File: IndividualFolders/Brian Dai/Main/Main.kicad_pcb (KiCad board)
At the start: 4 copper layers, 76.2 x 67.6 mm, 77 parts, among them J1 USB_B_Micro, J3 Conn_01x03, J4 Conn_01x03, J5 Conn_01x03, J6 Conn_01x03, SW1 SW_Push, SW2 SW_Push, U1 RP2350A-QFN60, U10 LM75B, U11 MCS1802GS-50-Z, U12 MCS1802GS-50-Z, U13 MCS1802GS-50-Z, U14 LM2575-3.3BT, U2 W25Q128JVS, U3 AMS1117-3.3, U4 MMC5983MA, U5 ICM-42688-P, U6 INA226, U7 KX134-1211, U8 MS5611-01BA, U9 MCS1802GS-50-Z, Y1 ABM8-272-T3

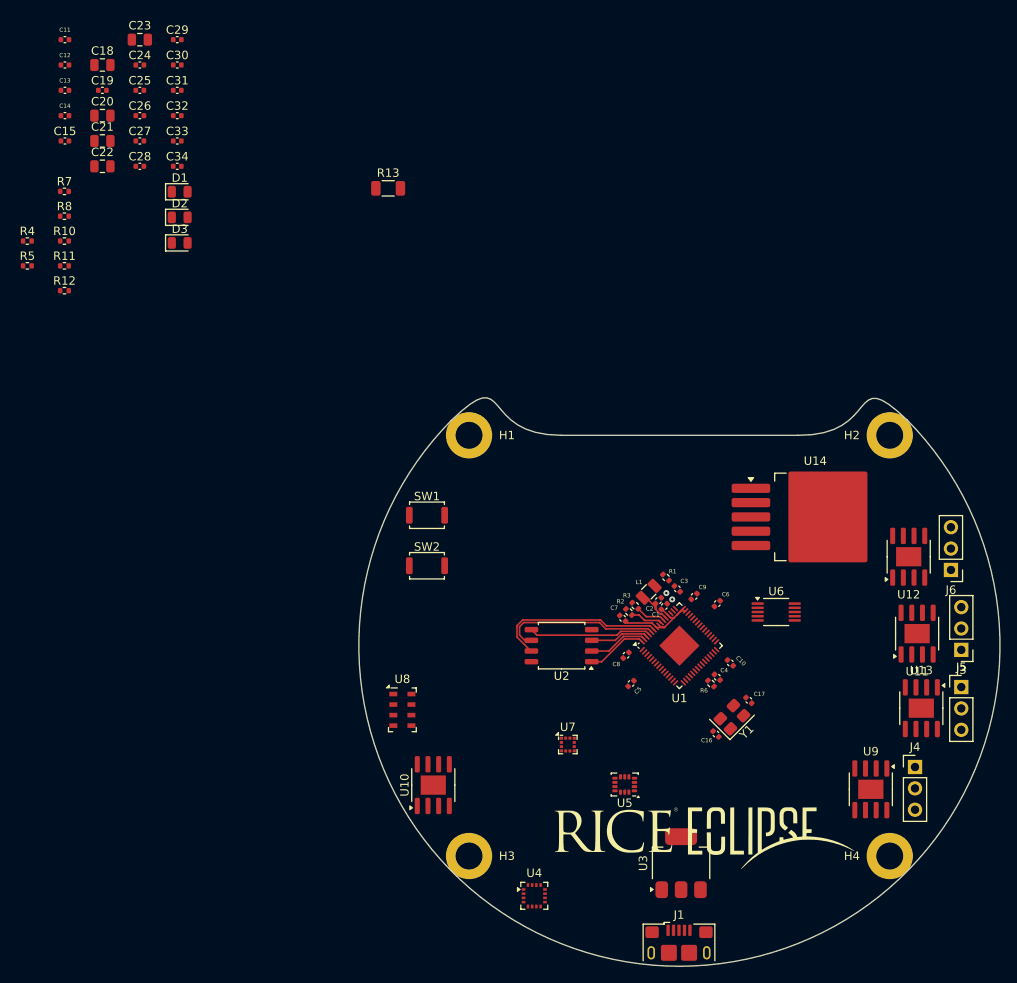
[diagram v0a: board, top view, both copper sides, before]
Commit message: Meeting 2/28/26
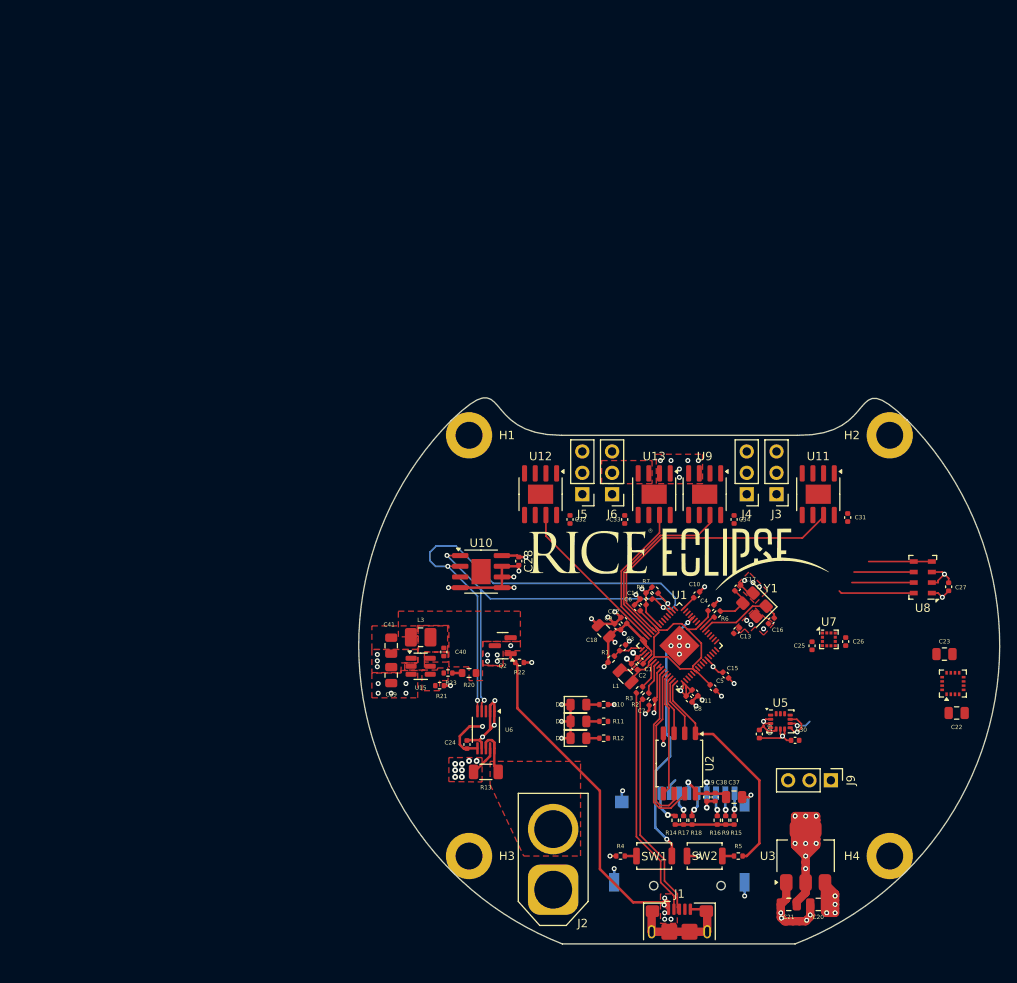
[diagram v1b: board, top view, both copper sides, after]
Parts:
- removed U14: LM2575-3.3BT, Package_TO_SOT_SMD:TO-263-5_TabPin3
- added C37: 10u, Capacitor_SMD:C_0805_2012Metric, F.Cu at (106.5, 118.0)
- added C38: 100n, Capacitor_SMD:C_0402_1005Metric, F.Cu at (104.2, 118.0)
- added C39: 10u, Capacitor_SMD:C_0805_2012Metric, F.Cu at (65.8, 103.5)
- added C40: 100n, Capacitor_SMD:C_0402_1005Metric, F.Cu at (72.0, 100.8)
- added C41: 22u, Capacitor_SMD:C_0805_2012Metric, F.Cu at (65.8, 100.0)
- added J2: XT60, Connector_AMASS:AMASS_XT60-M_1x02_P7.20mm_Vertical, F.Cu at (85.0, 129.0)
- added J7: MSD-4-A, otherComponents:CUI_MSD-4-A, B.Cu at (100.0, 125.3)
- added J9: Conn_01x03, Connector_PinHeader_2.54mm:PinHeader_1x03_P2.54mm_Vertical, F.Cu at (118.0, 116.0)
- added L3: 3.3u, Inductor_SMD:L_1008_2520Metric_Pad1.43x2.20mm_HandSolder, F.Cu at (69.2, 99.0)
- added Q2: Si2301CDS, Package_TO_SOT_SMD:SOT-23, F.Cu at (79.0, 100.0)
- added R14: 10k, Resistor_SMD:R_0402_1005Metric, F.Cu at (99.5, 120.8)
- added R15: 10k, Resistor_SMD:R_0402_1005Metric, F.Cu at (106.5, 120.8)
- added R16: 10k, Resistor_SMD:R_0402_1005Metric, F.Cu at (104.5, 120.8)
- added R17: 10k, Resistor_SMD:R_0402_1005Metric, F.Cu at (100.5, 120.8)
- added R18: 10k, Resistor_SMD:R_0402_1005Metric, F.Cu at (101.5, 120.8)
- added R20: 30k, Resistor_SMD:R_0603_1608Metric, F.Cu at (75.0, 103.2)
- added R21: 10k, Resistor_SMD:R_0402_1005Metric, F.Cu at (71.5, 104.8)
- added R22: 100k, Resistor_SMD:R_0402_1005Metric, F.Cu at (81.0, 102.0)
- added R23: 1k, Resistor_SMD:R_0402_1005Metric, F.Cu at (72.5, 103.2)
- added R9: 10k, Resistor_SMD:R_0402_1005Metric, F.Cu at (105.5, 120.8)
- added U15: AP62150WU, Package_TO_SOT_SMD:TSOT-23-6, F.Cu at (69.2, 102.5)
- D1: value LED -> RED_LED
- D2: value LED -> BLUE_LED
- D3: value LED -> GREEN_LED
- moved C20 126.6 mm to (116.5, 130.8), turned to 180 degrees
- moved C21 122.0 mm to (113.0, 130.8), turned to 180 degrees
- moved C22 120.5 mm to (132.9, 108.0), turned to 180 degrees
- moved C23 120.3 mm to (131.5, 101.0)
- moved C19 110.5 mm to (103.2, 118.0), turned to -90 degrees
- moved R5 109.8 mm to (107.0, 125.0)
- moved C27 109.8 mm to (132.0, 93.0), turned to 90 degrees
- moved C30 108.8 mm to (113.8, 111.2), turned to 180 degrees
- moved C11 107.8 mm to (101.8, 105.6), turned to -45 degrees
- moved C29 107.7 mm to (109.5, 110.5), turned to -90 degrees
- moved C26 104.6 mm to (119.8, 99.5), turned to -90 degrees
- moved C25 103.6 mm to (115.8, 100.0), turned to -90 degrees
- moved C13 102.4 mm to (106.8, 98.2), turned to 45 degrees
- moved R4 101.5 mm to (93.0, 125.0)
- moved C15 101.0 mm to (105.5, 103.5), turned to -45 degrees
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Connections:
- C29 pad 2: Net-(C29-Pad2) -> GND
- C30 pad 2: Net-(C29-Pad2) -> GND
- R13 pad 1: GND -> VIN
- R13 pad 2: VSS -> Net-(J2-Pin_2)
- U1 pad 24: unconnected-(U1-SWCLK-Pad24) -> Net-(J9-Pin_3)
- U1 pad 25: unconnected-(U1-SWDIO-Pad25) -> Net-(J9-Pin_2)
- U1 pad 32: unconnected-(U1-GPIO20-Pad32) -> SDA
- U1 pad 33: unconnected-(U1-GPIO21-Pad33) -> SCL
- U1 pad 40: unconnected-(U1-GPIO26_ADC0-Pad40) -> Vout1
- U1 pad 41: unconnected-(U1-GPIO27_ADC1-Pad41) -> Vout2
- U1 pad 42: unconnected-(U1-GPIO28_ADC2-Pad42) -> Vout4
- U1 pad 43: unconnected-(U1-GPIO29_ADC3-Pad43) -> Vout3
- U11 pad 1: current + -> VIN
- U11 pad 2: current + -> VIN
- U12 pad 3: current + -> VIN
- U12 pad 4: current + -> VIN
- U13 pad 1: current + -> VIN
- U13 pad 2: current + -> VIN
- U6 pad 10: VSS -> Net-(J2-Pin_2)
- U6 pad 8: GND -> Net-(J2-Pin_2)
- U6 pad 9: GND -> VIN
- U7 pad 1: ACCEL_SDO/ADDR -> SPI_SD0
- U7 pad 2: ACCEL_SDI/SDA -> SPI_SDI
- U9 pad 3: current + -> VIN
- U9 pad 4: current + -> VIN
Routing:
- net GND: track 0.18 -> 105.7 mm, vias 2 -> 55
- net +3.3V: track 12.1 -> 104.9 mm, vias 0 -> 27
- net SCL: track 0.00 -> 61.0 mm, vias 0 -> 3
- net VBUS: track 0.00 -> 56.0 mm, vias 0 -> 9
- net SDA: track 0.00 -> 48.2 mm, vias 0 -> 3
- net Vout1: track 0.00 -> 34.6 mm
- net Net-(U1-RUN): track 0.00 -> 31.4 mm, vias 0 -> 2
- net +1V1: track 4.52 -> 34.6 mm
- net /USB_D-: track 0.00 -> 27.6 mm
- net /USB_D+: track 0.00 -> 27.0 mm
- net Vout2: track 0.00 -> 22.1 mm
- net /QSPI_SS: track 7.25 -> 27.3 mm
- net Vout3: track 0.00 -> 19.5 mm
- net Vout4: track 0.00 -> 17.5 mm
- net Net-(U1-XIN): track 0.00 -> 10.3 mm
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- added copper zone on F.Cu, net +3.3V
- added copper zone on In2.Cu, net +3.3V
- added copper zone on F.Cu, net GND
- added copper zone on In1.Cu, net GND
- added copper zone on F.Cu, net Net-(J2-Pin_2)
- added copper zone on F.Cu, net Net-(Q2-S)
- added copper zone on F.Cu, net Net-(U15-BST)
- added copper zone on F.Cu, net Net-(U15-FB)
- added copper zone on F.Cu, net Net-(U15-SW)
- added copper zone on F.Cu, net VBUS
- added copper zone on In2.Cu, net VBUS
- added copper zone on F.Cu, net VIN
- added copper zone on In2.Cu, net VIN
- added copper zone on F.Cu, net current -4
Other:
- board size 76.2 x 67.6 mm -> 76.2 x 64.9 mm
- board text added: "SIG, GND, PWR, SIG Stackup"
